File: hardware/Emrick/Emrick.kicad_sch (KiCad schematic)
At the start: 88 parts, among them J1 LED_STRIP_CONNECTOR, J2 UFL, J3 Conn_02x05_Odd_Even, J4 BATT_CONN, P1 USB_C_Plug_USB2.0, Q1 Q_NMOS_GSD, Q2 Q_NMOS_GSD, Q3 Q_NMOS_GSD, SW1 SW_SPST, SW2 SW_MEC_5E (RESET), U1 74HCT541, U2 CC1310, U3 TPS63020, U4 CP2102N, U5 MX25R8035F, U6 BQ24072, Y1 24MHz, Y2 32.768kHz

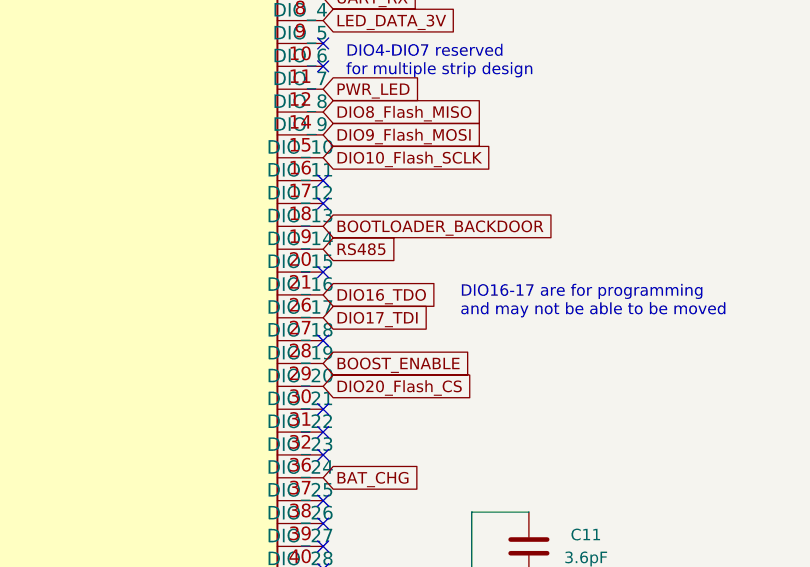
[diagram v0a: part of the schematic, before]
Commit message: revision 2
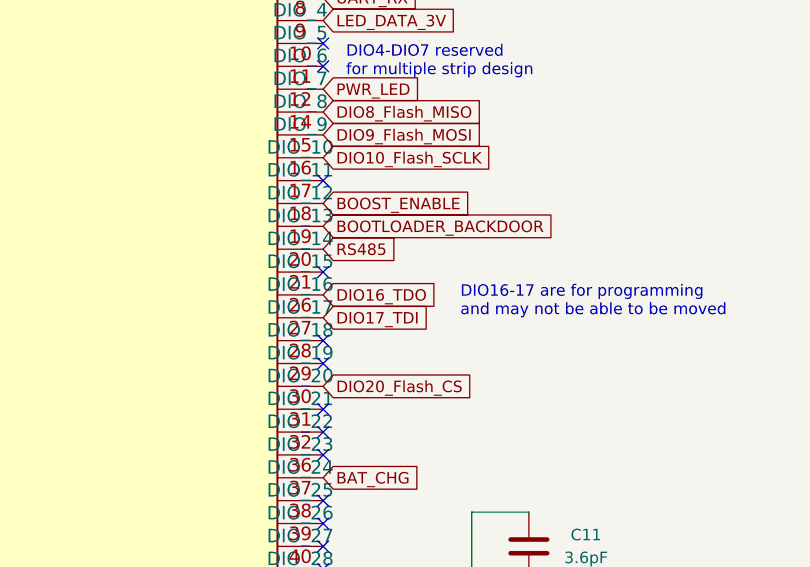
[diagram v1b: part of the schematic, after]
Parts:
- C12: footprint Capacitor_SMD:C_0201_0603Metric -> Capacitor_SMD:C_0402_1005Metric
- C13: footprint Capacitor_SMD:C_0201_0603Metric -> Capacitor_SMD:C_0603_1608Metric
- C29: footprint Capacitor_SMD:C_0402_1005Metric -> Capacitor_SMD:C_0603_1608Metric
- L9: footprint Inductor_SMD:L_0402_1005Metric -> Capacitor_SMD:C_0603_1608Metric
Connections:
- net BOOST_ENABLE: now also U2.18 (DIO_12); no longer U2.29 (DIO_19)
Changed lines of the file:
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@@
   (junction (at 292.1 255.27) (diameter 0) (color 0 0 0 0)
   )
+  (no_connect (at 217.17 83.82))
   (no_connect (at 158.75 248.92))
   (no_connect (at 158.75 256.54))
@@
   (no_connect (at 62.23 40.64))
   (no_connect (at 217.17 63.5))
-  (no_connect (at 217.17 66.04))
+  (no_connect (at 217.17 88.9))
   (no_connect (at 217.17 38.1))
   (no_connect (at 217.17 91.44))
@@
   (no_connect (at 45.72 172.72))
   (no_connect (at 217.17 106.68))
-  (no_connect (at 217.17 88.9))
   (no_connect (at 217.17 104.14))
   (no_connect (at 217.17 101.6))
@@
     )
   )
-  (global_label "BOOST_ENABLE" (shape input) (at 217.17 83.82 0) (fields_autoplaced)
+  (global_label "BOOST_ENABLE" (shape input) (at 217.17 66.04 0) (fields_autoplaced)
     (effects (font (size 1.27 1.27)) (justify left))
-    (property "Intersheet References" "${INTERSHEET_REFS}" (id 0) (at 233.6741 83.7406 0)
+    (property "Intersheet References" "${INTERSHEET_REFS}" (id 0) (at 233.6741 65.9606 0)
       (effects (font (size 1.27 1.27)) (justify left) hide)
     )
@@
       (effects (font (size 1.27 1.27)) (justify left))
     )
-    (property "Footprint" "Inductor_SMD:L_0402_1005Metric" (id 2) (at 320.04 125.73 0)
+    (property "Footprint" "Capacitor_SMD:C_0603_1608Metric" (id 2) (at 320.04 125.73 0)
       (effects (font (size 1.27 1.27)) hide)
     )
@@
       (effects (font (size 1.27 1.27)) (justify left))
     )
-    (property "Footprint" "Capacitor_SMD:C_0201_0603Metric" (id 2) (at 287.9852 109.22 0)
+    (property "Footprint" "Capacitor_SMD:C_0402_1005Metric" (id 2) (at 287.9852 109.22 0)
       (effects (font (size 1.27 1.27)) hide)
     )
@@
       (effects (font (size 1.27 1.27)) (justify left))
     )
-    (property "Footprint" "Capacitor_SMD:C_0201_0603Metric" (id 2) (at 312.1152 129.54 0)
+    (property "Footprint" "Capacitor_SMD:C_0603_1608Metric" (id 2) (at 312.1152 129.54 0)
       (effects (font (size 1.27 1.27)) hide)
     )
@@
       (effects (font (size 1.27 1.27)) (justify right))
     )
-    (property "Footprint" "Capacitor_SMD:C_0402_1005Metric" (id 2) (at 386.3848 205.74 0)
+    (property "Footprint" "Capacitor_SMD:C_0603_1608Metric" (id 2) (at 386.3848 205.74 0)
       (effects (font (size 1.27 1.27)) hide)
     )
@@
     )
     (path "/4f3938ec-ee10-4033-b043-17e527f7cafe"
-      (reference "C12") (unit 1) (value "?") (footprint "Capacitor_SMD:C_0201_0603Metric")
+      (reference "C12") (unit 1) (value "?") (footprint "Capacitor_SMD:C_0402_1005Metric")
     )
     (path "/50c8f597-eecd-41b3-b369-057fd39f4039"
-      (reference "C13") (unit 1) (value "?") (footprint "Capacitor_SMD:C_0201_0603Metric")
+      (reference "C13") (unit 1) (value "?") (footprint "Capacitor_SMD:C_0603_1608Metric")
     )
     (path "/2b92eedf-d2a7-4ca6-a1c8-41794a417b5e"
@@
     )
     (path "/80b7865e-df93-429c-94a4-4f595f2b7920"
-      (reference "C29") (unit 1) (value "10uF") (footprint "Capacitor_SMD:C_0402_1005Metric")
+      (reference "C29") (unit 1) (value "10uF") (footprint "Capacitor_SMD:C_0603_1608Metric")
     )
     (path "/0c17f3c6-00d6-4552-8d5c-ffe417b95235"
@@
     )
     (path "/3240c5b7-b3f1-4039-96ce-b8816fd0780e"
-      (reference "L9") (unit 1) (value "?") (footprint "Inductor_SMD:L_0402_1005Metric")
+      (reference "L9") (unit 1) (value "?") (footprint "Capacitor_SMD:C_0603_1608Metric")
     )
     (path "/98b2397c-2d8e-4422-bb18-42d4b4daae2e"
